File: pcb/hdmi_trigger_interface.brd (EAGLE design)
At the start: 78.7 x 63.5 mm, 58 parts, among them U1 TPD12S016PWR, U2 TPD12S016PWR, Y1 SI514

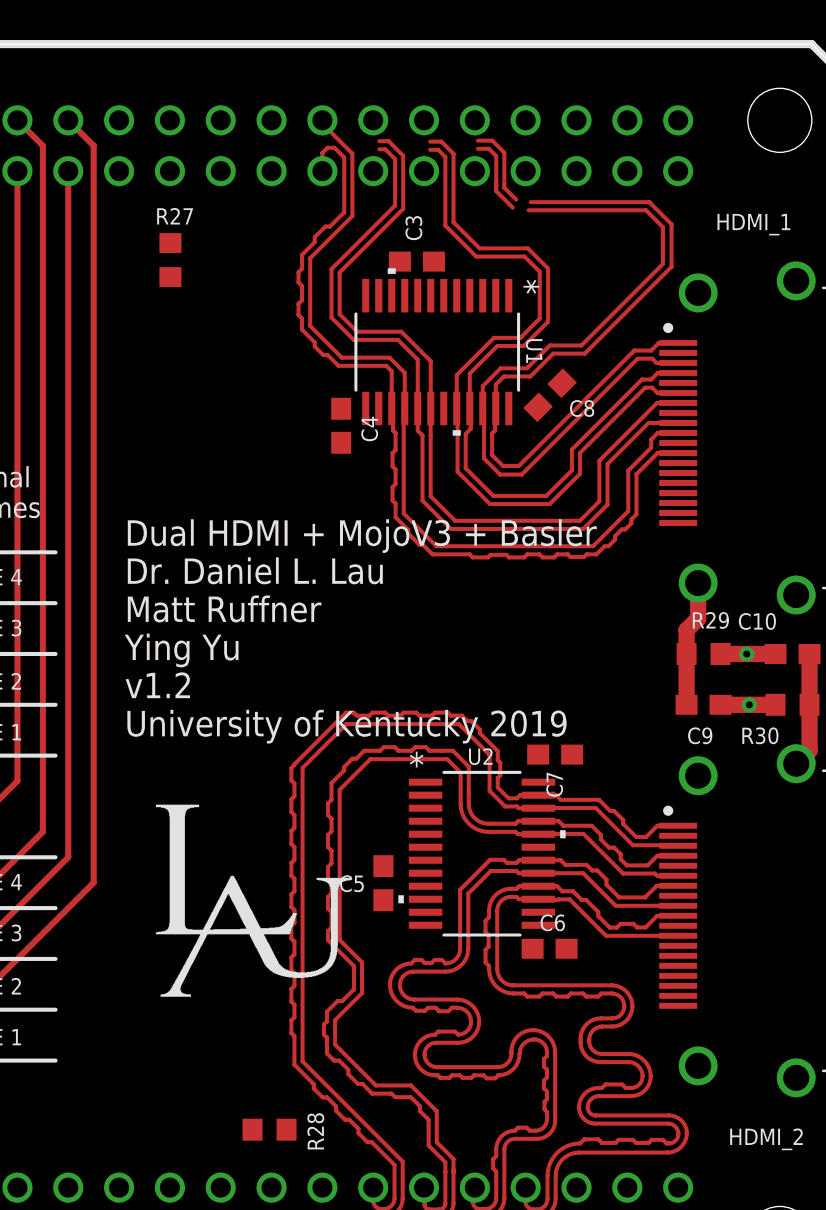
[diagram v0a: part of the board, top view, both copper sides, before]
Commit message: more work on length tuning
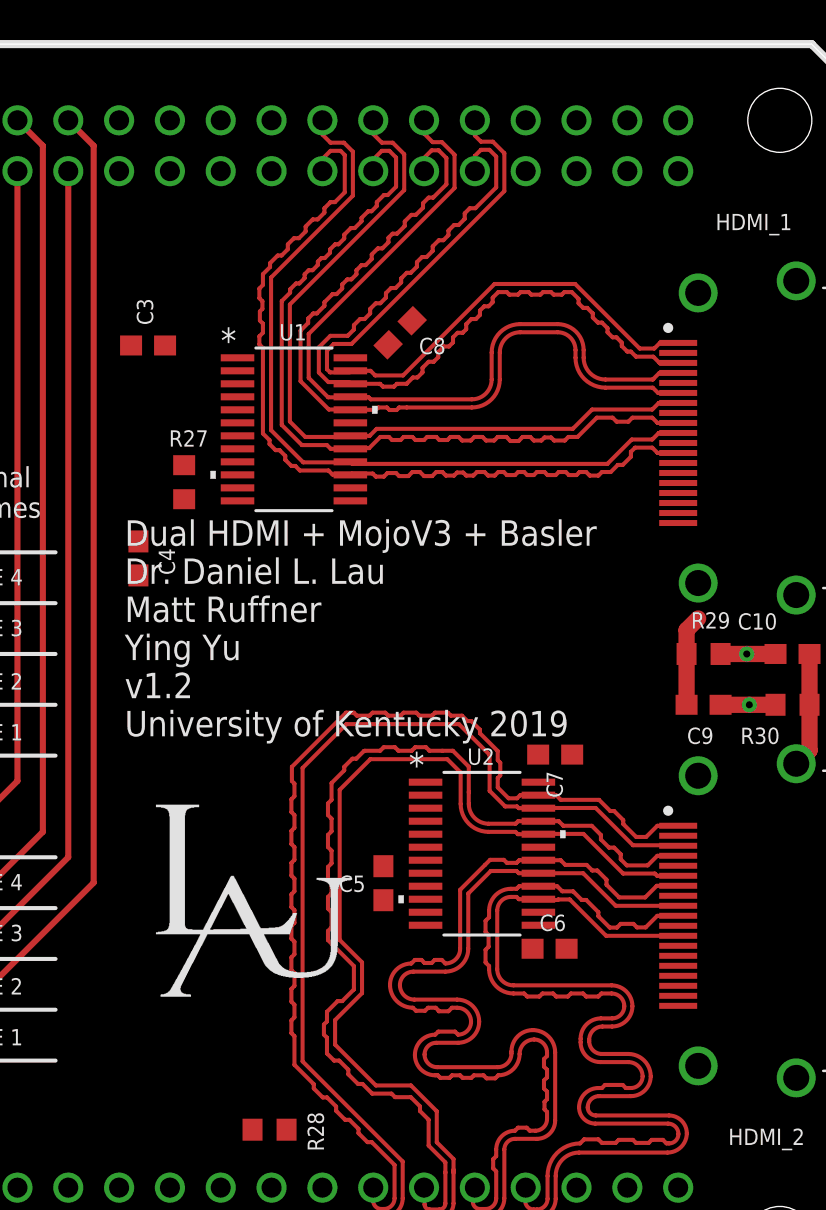
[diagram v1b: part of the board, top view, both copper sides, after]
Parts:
- moved C3 14.1 mm to (43.4, 48.4)
- moved C4 12.1 mm to (42.9, 37.8)
- moved R27 11.1 mm to (45.2, 41.6)
- moved U1 8.14 mm to (50.6, 44.2), turned to 0 degrees
- moved C8 8.12 mm to (56.0, 49.1)
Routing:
- net D11_N: track 37.3 -> 41.5 mm
- net CLK1_P: track 42.7 -> 39.9 mm
- net D11_P: track 37.4 -> 39.6 mm
- net D21_P: track 40.7 -> 38.6 mm
- net N$13: track 6.33 -> 4.55 mm
- net CLK1_N: track 44.3 -> 42.7 mm
- net D01_N: track 39.5 -> 40.9 mm
- net D01_P: track 39.5 -> 38.8 mm
- net D21_N: track 40.7 -> 41.4 mm

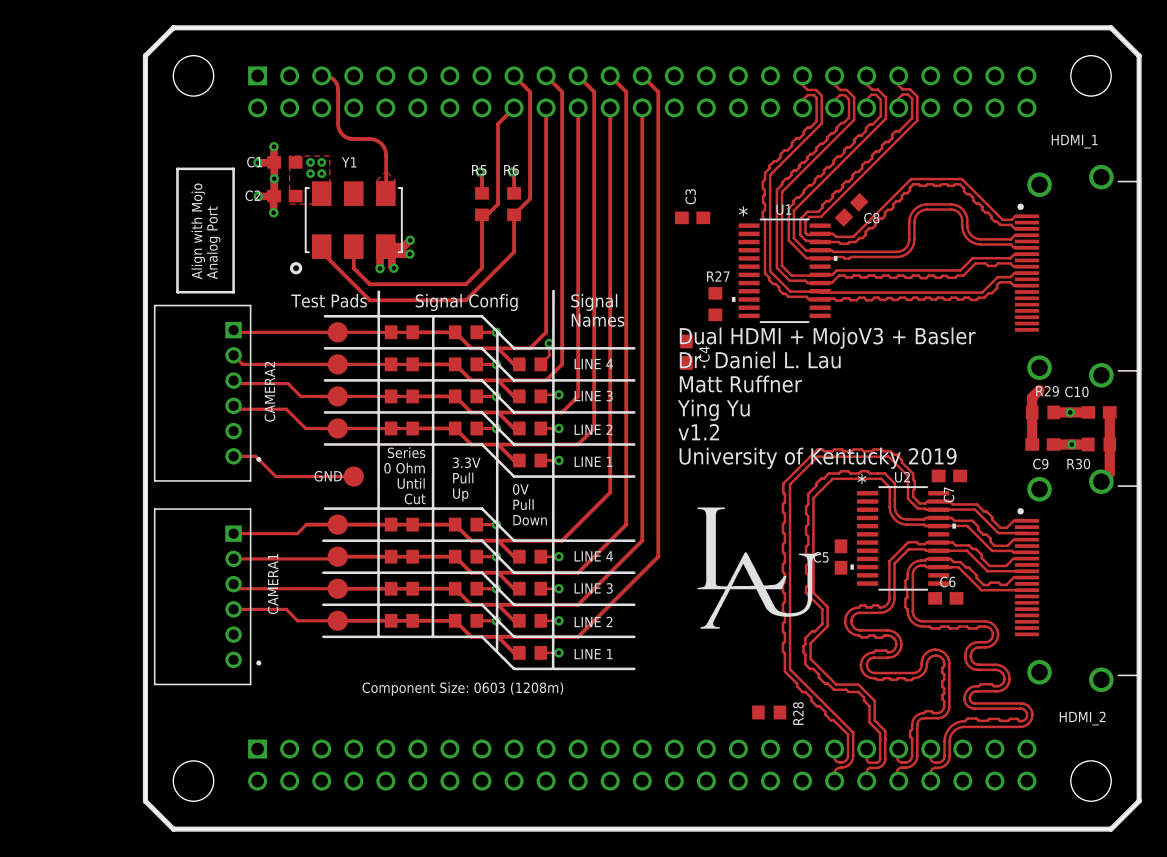
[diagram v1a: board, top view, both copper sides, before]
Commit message: more routing
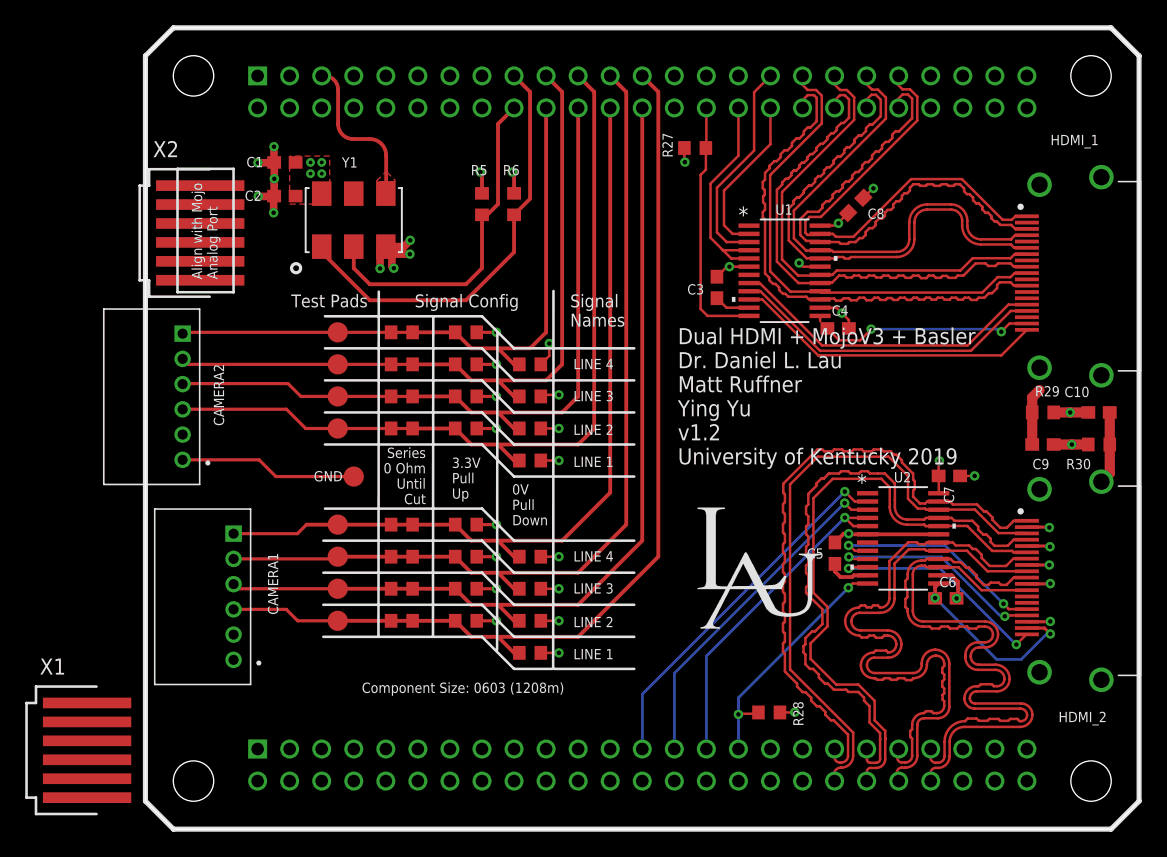
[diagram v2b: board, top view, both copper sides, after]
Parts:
- added X1, X2: 87438-06, con-molex:87438-06
- moved R27 12.5 mm to (43.6, 54.0), turned to 0 degrees
- moved C4 12.2 mm to (54.9, 39.7), turned to 0 degrees
- moved C3 5.84 mm to (45.3, 42.9), turned to 90 degrees
- moved CAMERA2 4.05 mm to (2.95, 34.3)
- moved C5 0.57 mm to (54.6, 21.9)
- moved C8 0.49 mm to (56.3, 49.4)
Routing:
- net GND: track 43.9 -> 79.1 mm, vias 19 -> 31
- net SCL2_M: track 0.00 -> 29.2 mm, vias 0 -> 1
- net SDA2_M: track 0.00 -> 27.1 mm, vias 0 -> 1
- net HP2_M: track 0.00 -> 26.7 mm, vias 0 -> 1
- net SCL1: track 0.00 -> 25.4 mm
- net SDA1: track 0.00 -> 25.3 mm
- net HP1: track 0.00 -> 24.7 mm
- net CTHPD1: track 0.06 -> 20.2 mm
- net CTHPD2: track 0.14 -> 19.7 mm, vias 0 -> 2
- net HP2: track 0.00 -> 18.6 mm, vias 0 -> 2
- net SCL2: track 0.00 -> 17.9 mm, vias 0 -> 2
- net SDA2: track 0.00 -> 17.7 mm, vias 0 -> 2
- net 5VHDMI1: track 0.00 -> 17.5 mm, vias 0 -> 2
- net HP1_M: track 0.00 -> 17.0 mm
- net SDA1_M: track 0.00 -> 17.0 mm
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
